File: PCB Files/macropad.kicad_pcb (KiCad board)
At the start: 2 copper layers, 73.3 x 70.1 mm, 7 parts, among them SW1 SW_Push, SW2 SW_Push, SW3 SW_Push, SW5 SW_Push, U1 MOUDLE-SEEEDUINO-XIAO, U3 ER_OLEDM0.91_1x-I2C

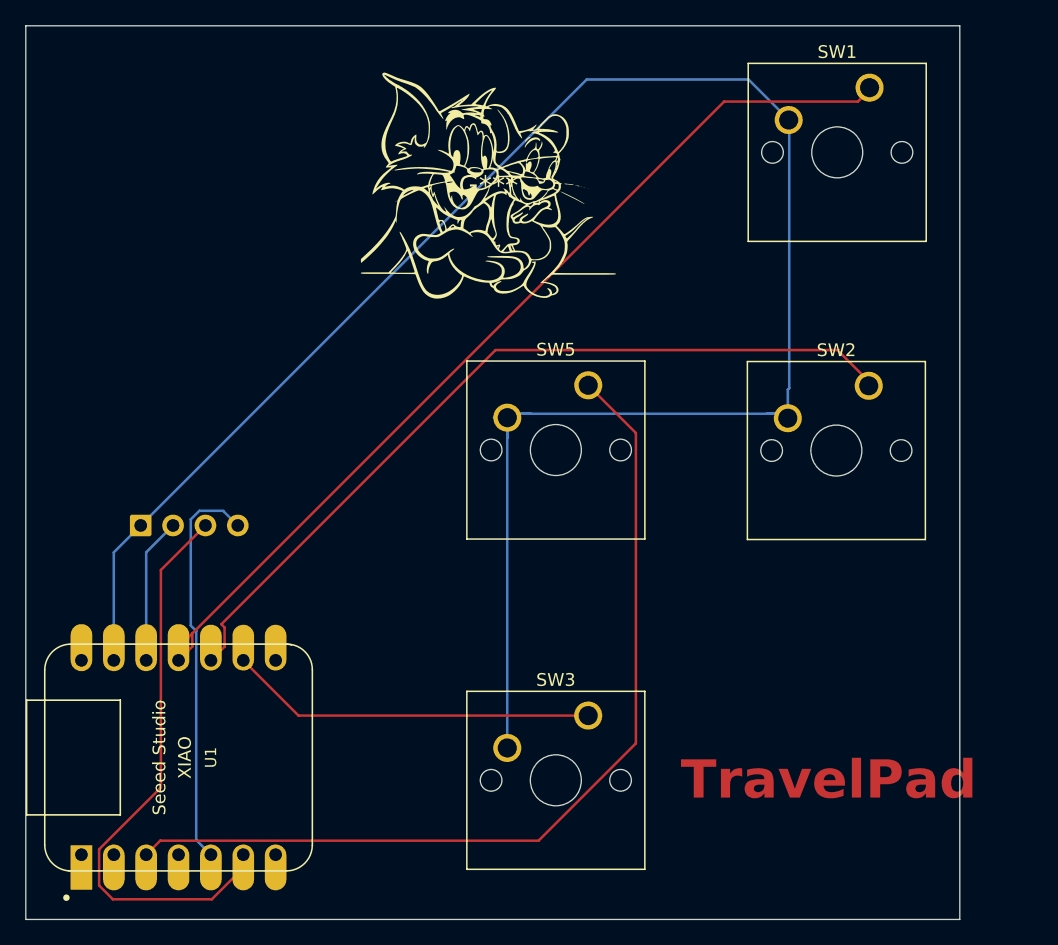
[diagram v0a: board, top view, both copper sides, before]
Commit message: Add files via upload
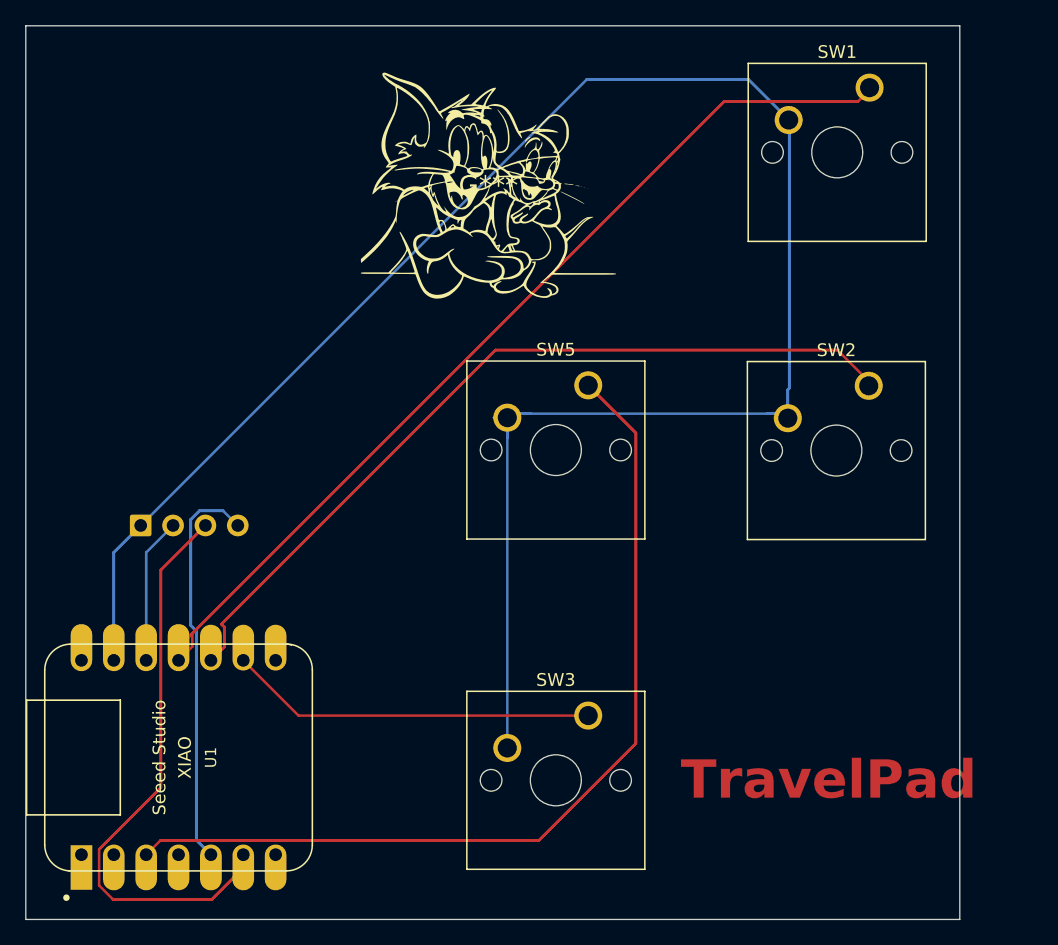
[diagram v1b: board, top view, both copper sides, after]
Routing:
- net Net-(U1-PA6_A10_D10_MOSI): track 76.9 -> 149.6 mm
- net Net-(U1-PA10_A2_D2): track 71.7 -> 141.8 mm
- net Net-(U1-PA5_A9_D9_MISO): track 64.2 -> 125.0 mm
- net GND: track 156.4 -> 215.8 mm
- net Net-(U1-PA9_A5_D5_SCL): track 45.7 -> 86.9 mm
- net Net-(U1-PA8_A4_D4_SDA): track 31.4 -> 61.2 mm
